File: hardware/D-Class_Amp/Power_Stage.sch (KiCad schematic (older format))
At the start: 16 parts

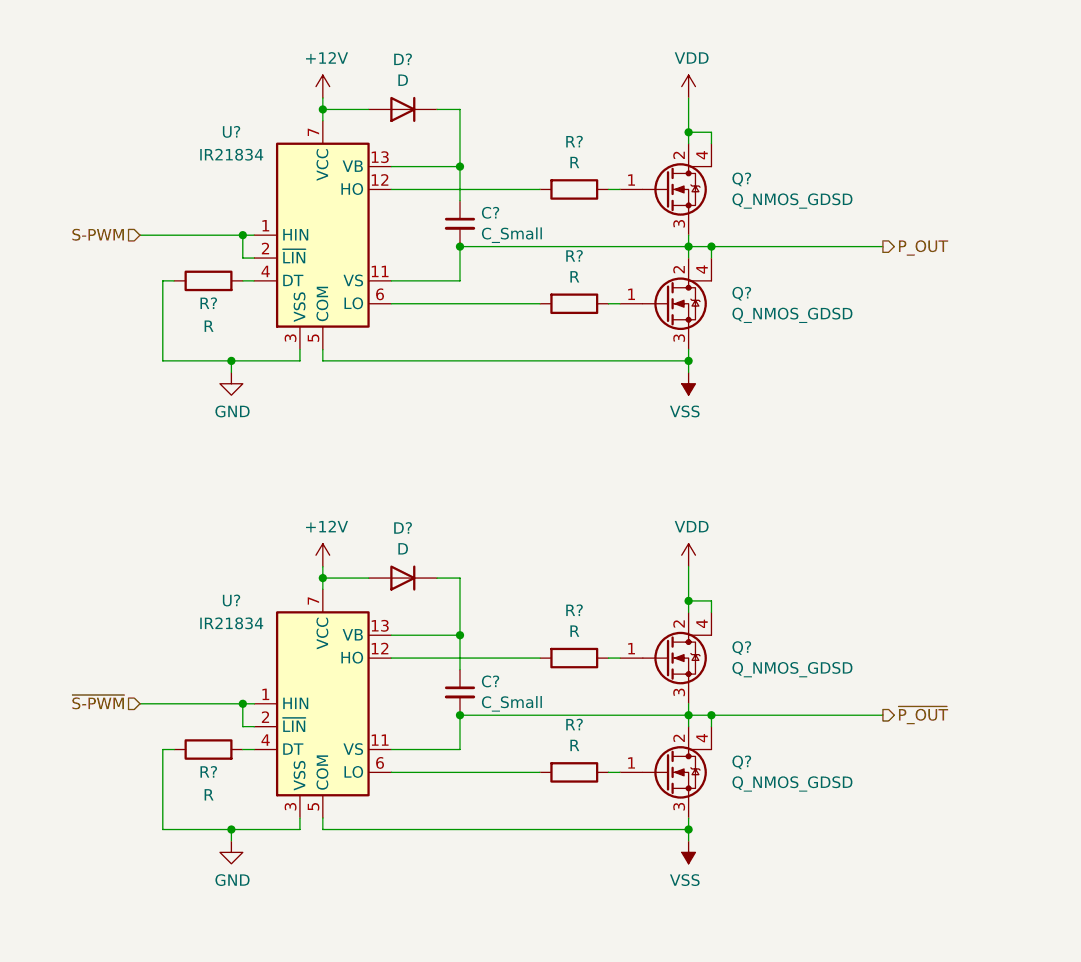
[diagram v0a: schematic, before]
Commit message: anot
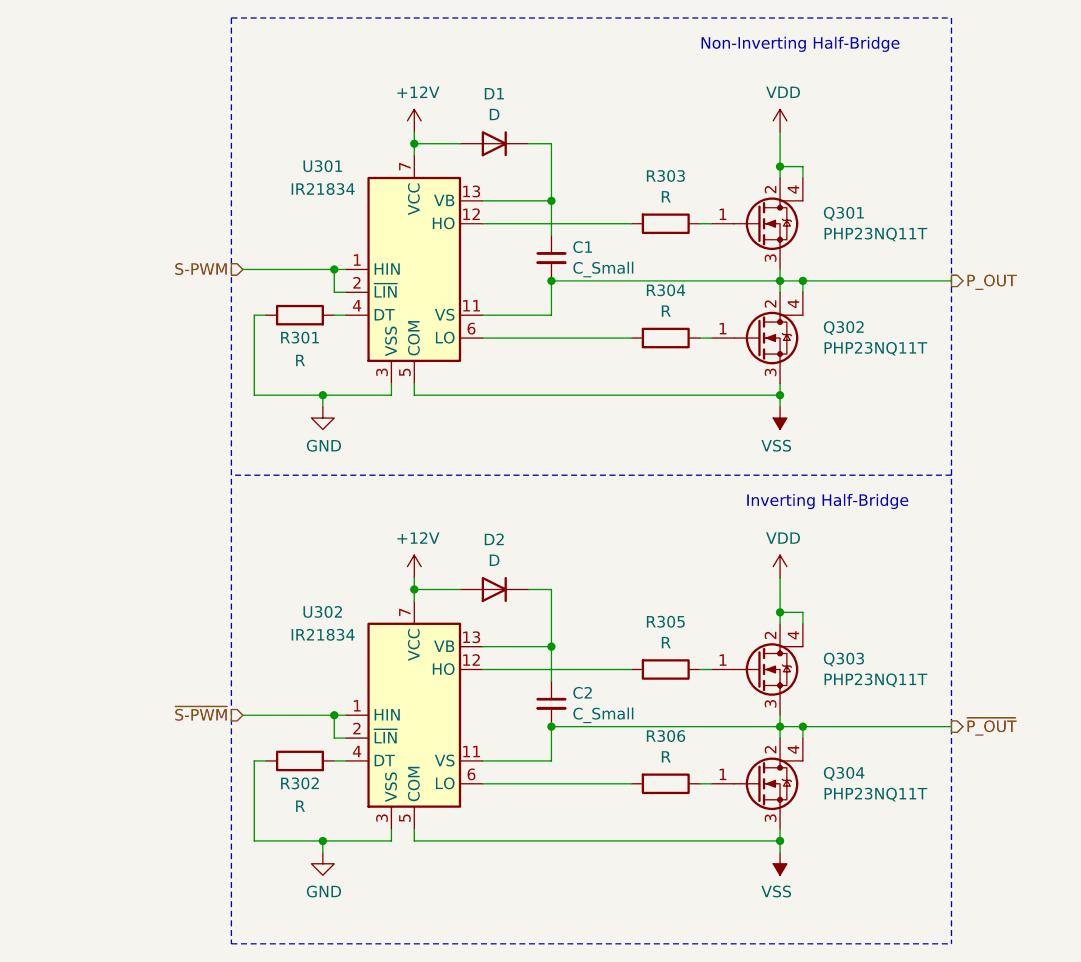
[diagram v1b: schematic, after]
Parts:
- Q301, Q302, Q303, Q304: renamed from Q?; value Q_NMOS_GDSD -> PHP23NQ11T
- gave numbers to parts that had none: 12
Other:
- note added: "Inverting Half-Bridge\n"
- note added: "Non-Inverting Half-Bridge\n"
- moved on the sheet: C1, C2, D1, D2, Q301, Q302, Q303, Q304, R301, R302, R303, R304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
